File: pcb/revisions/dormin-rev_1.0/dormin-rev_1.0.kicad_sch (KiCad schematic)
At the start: 70 parts, among them SW1 SW_PUSH-MX_CHOC, SW10 SW_PUSH-MX_CHOC, SW11 SW_PUSH-MX_CHOC, SW12 SW_PUSH-MX_CHOC, SW13 SW_PUSH-MX_CHOC, SW14 SW_PUSH-MX_CHOC, SW15 SW_PUSH-MX_CHOC, SW16 SW_PUSH-MX_CHOC, SW17 SW_PUSH-MX_CHOC, SW19 SW_PUSH-MX_CHOC, SW2 SW_PUSH-MX_CHOC, SW20 SW_PUSH-MX_CHOC, SW21 SW_PUSH-MX_CHOC, SW22 SW_PUSH-MX_CHOC, SW3 SW_PUSH-MX_CHOC, SW4 SW_PUSH-MX_CHOC, SW5 SW_PUSH-MX_CHOC, SW6 SW_PUSH-MX_CHOC, SW7 SW_PUSH-MX_CHOC, SW8 SW_PUSH-MX_CHOC, SW9 SW_PUSH-MX_CHOC, U1 Seeeduino Xiao nRF52840

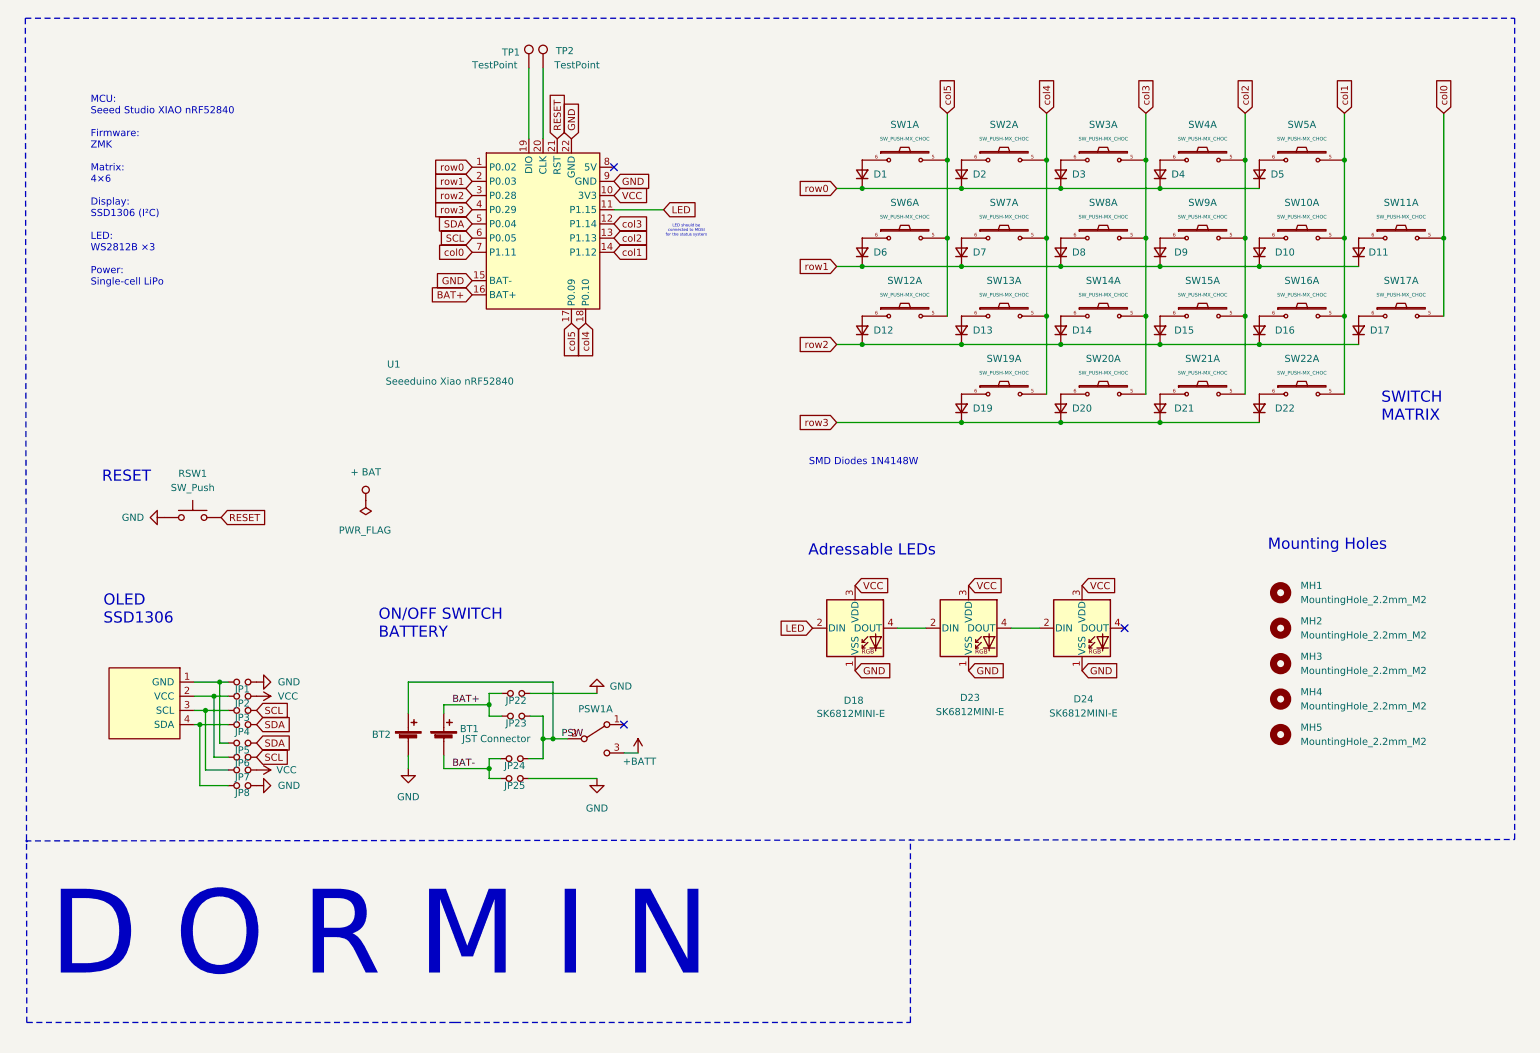
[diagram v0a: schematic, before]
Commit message: refactor: added initial versions of the pcb
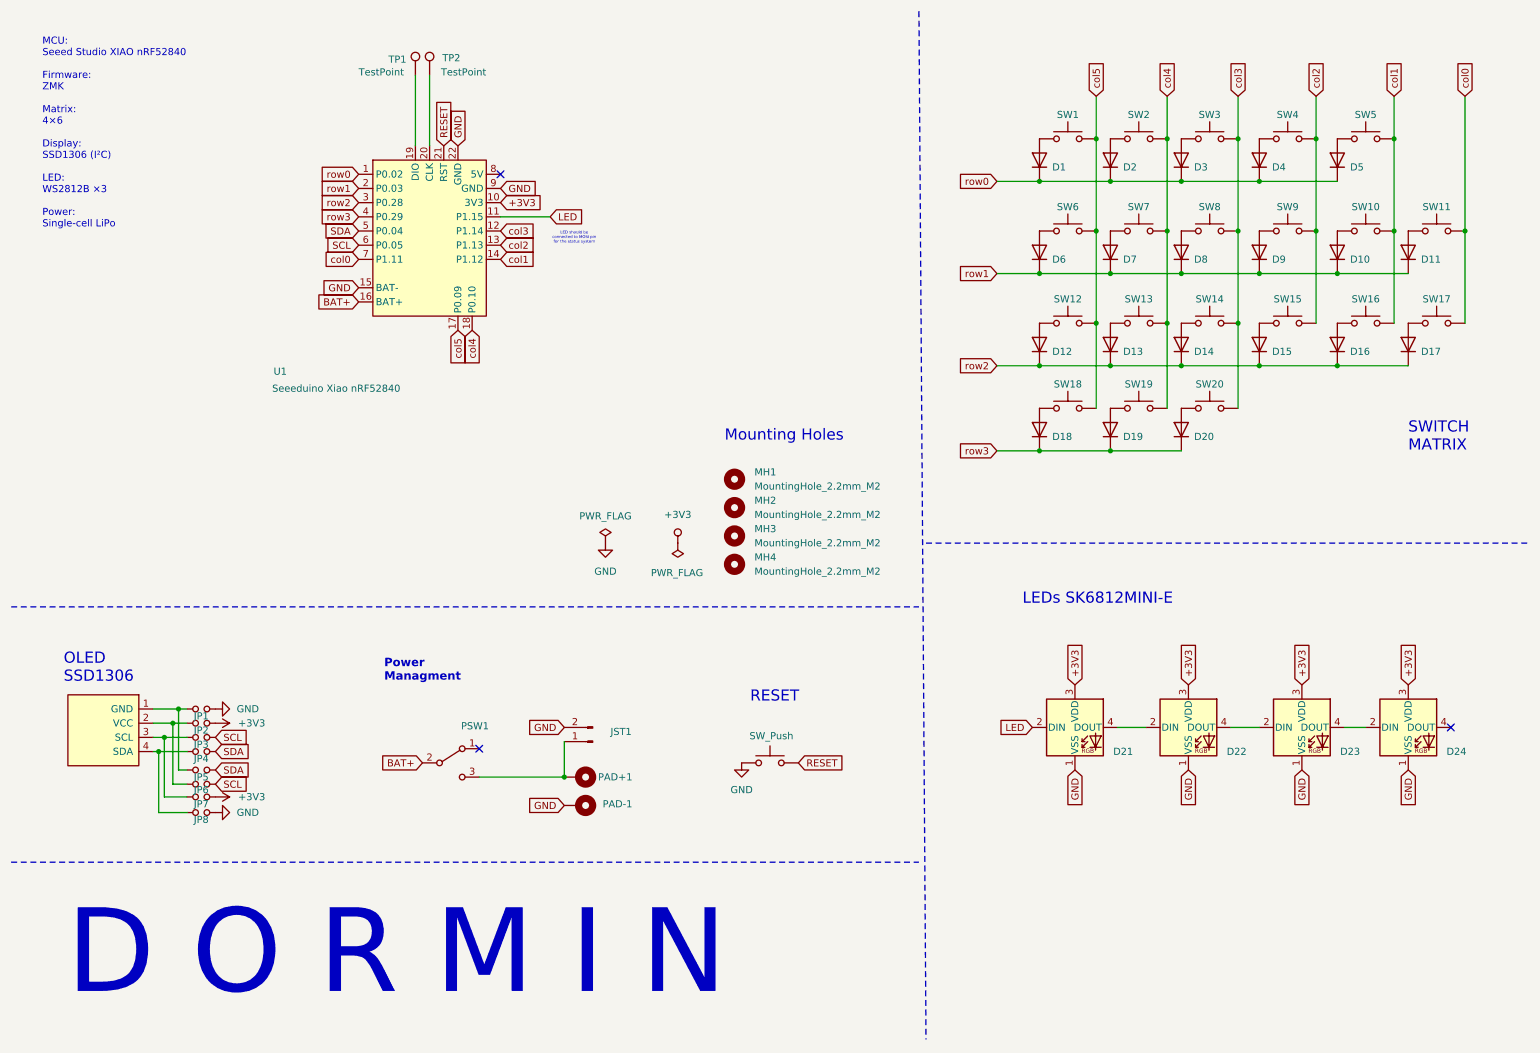
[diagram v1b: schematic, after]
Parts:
- removed BT1: JST Connector, KLOR:JST_PH_reversible, symbol Device:Battery_Cell
- removed BT2: Battery_Cell, KLOR:custombatteryconnector_small, symbol Device:Battery_Cell
- removed D1, D10, D11, D12, D13, D14, D15, D16, D17, D19, D2, D20, D21, D22, D3, D4, D5, D6, D7, D8, D9: D_Small, KLOR:Diode_SOD123, symbol Device:D_Small
- removed D18: SK6812MINI-E, LED_SMD:LED_SK6812MINI-E_3.2x2.8mm_P1.5mm_ReverseMount, symbol LED:SK6812MINI-E
- removed JP22, JP23, JP24, JP25: Device_Jumper_NO_Small, KLOR:Jumper, symbol KLORlib:Device_Jumper_NO_Small
- removed MH5: MountingHole_2.2mm_M2, MountingHole:MountingHole_2.2mm_M2, symbol Mechanical:MountingHole
- removed PSW1: SW_DPDT_x2, KLOR:MSK12C02_reversible, symbol Switch:SW_DPDT_x2
- removed SW1, SW10, SW11, SW12, SW13, SW14, SW15, SW16, SW17, SW19, SW2, SW20, SW21, SW22, SW3, SW4, SW5, SW6, SW7, SW8, SW9: SW_PUSH-MX_CHOC, WillKeebs_Kicad_Gateron:SW_MXchoc_HS_1u, symbol KLORlib:SW_PUSH-MX_W_LED
- added D1, D10, D11, D12, D13, D14, D15, D16, D17, D18, D19, D2, D20, D3, D4, D5, D6, D7, D8, D9: 1N4148W, Diode_SMD:D_SOD-123, symbol Diode:1N4148W
- added D21, D22: SK6812MINI-E, LED_SMD:LED_SK6812MINI-E_3.2x2.8mm_P1.5mm_ReverseMount, symbol LED:SK6812MINI-E
- added JST1: Conn_01x02_Pin, Connector_JST:JST_GH_SM02B-GHS-TB_1x02-1MP_P1.25mm_Horizontal, symbol Connector:Conn_01x02_Pin
- added PAD+1: +, ScottoKeebs_Scotto:Battery, symbol Mechanical:MountingHole_Pad
- added PAD-1: -, TOTEMlib:BatteryPad, symbol Mechanical:MountingHole_Pad
- added PSW1: SW_SPDT, Button_Switch_SMD:SW_SPDT_Shouhan_MSK12C02, symbol Switch:SW_SPDT
- added SW1, SW10, SW11, SW12, SW13, SW14, SW15, SW16, SW17, SW18, SW19, SW2, SW20, SW3, SW4, SW5, SW6, SW7, SW8, SW9: SW_Push, WillKeebs_Kicad_Gateron:SW_MXchoc_HS_1u, symbol Switch:SW_Push
- OLED1: footprint KLOR:SSD1306_128x64OLED -> ScottoKeebs_Components:OLED_128x32
- RSW1: footprint KLOR:SW_Push_1P1T-MP_NO_Horizontal_Alps_SKRTLAE010_both_sides -> Button_Switch_SMD:SW_Push_1P1T_XKB_TS-1187A
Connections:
- net BAT+: now also PSW1.2 (B)
- net GND: now also D21.1 (VSS), D22.1 (VSS), JST1.2 (Pin_2), PAD-1.1
- net LED: now also D21.2 (DIN)
- net col0: now also SW11.2, SW17.2
- net col1: now also SW10.2, SW16.2, SW5.2
- net col2: now also SW15.2, SW4.2, SW9.2
- net col3: now also SW14.2, SW20.2, SW3.2, SW8.2
- net col4: now also SW13.2, SW19.2, SW2.2, SW7.2
- net col5: now also SW1.2, SW12.2, SW18.2, SW6.2
- net row0: now also D1.1 (K), D2.1 (K), D3.1 (K), D4.1 (K), D5.1 (K)
- net row1: now also D10.1 (K), D11.1 (K), D6.1 (K), D7.1 (K), D8.1 (K), D9.1 (K)
- net row2: now also D12.1 (K), D13.1 (K), D14.1 (K), D15.1 (K), D16.1 (K), D17.1 (K)
- net row3: now also D18.1 (K), D19.1 (K), D20.1 (K)
- net at D23.2 (DIN): now also D22.4 (DOUT)
- net VCC renamed +3V3
- net +3V3: now also D21.3 (VDD), D22.3 (VDD)
- new net: D10.2 (A), SW10.1
- new net: D14.2 (A), SW14.1
- new net: D9.2 (A), SW9.1
- new net: D7.2 (A), SW7.1
- new net: D16.2 (A), SW16.1
- new net: D3.2 (A), SW3.1
- new net: D1.2 (A), SW1.1
- new net: D12.2 (A), SW12.1
- new net: D8.2 (A), SW8.1
- new net: D19.2 (A), SW19.1
- new net: D17.2 (A), SW17.1
- new net: D2.2 (A), SW2.1
- new net: D20.2 (A), SW20.1
- new net: D15.2 (A), SW15.1
- new net: D5.2 (A), SW5.1
- new net: D11.2 (A), SW11.1
- new net: D4.2 (A), SW4.1
- new net: JST1.1 (Pin_1), PAD+1.1, PSW1.3 (C)
- new net: D6.2 (A), SW6.1
- new net: D18.2 (A), SW18.1
- new net: D13.2 (A), SW13.1
- new net: D21.4 (DOUT), D22.2 (DIN)
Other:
- note added: "LED should be connected to MOSI pin for the status system"
- note added: "LEDs SK6812MINI-E"
- note added: "Power Managment"
- note removed: "Adressable LEDs"
- note removed: "LED should be connected to MOSI for the status system"
- note removed: "ON/OFF SWITCH BATTERY"
- note removed: "SMD Diodes 1N4148W"
- title: Dormin Split Keyboard -> Dormin Keyboard
